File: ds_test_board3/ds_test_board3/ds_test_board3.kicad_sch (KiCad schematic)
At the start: 126 parts, among them J1 DF40C-60DP-0.4V_51_, J2 DF40C-60DP-0.4V_51_, J3 Conn_01x30, J4 Conn_01x30, J5 Conn_01x30, J6 Conn_01x30

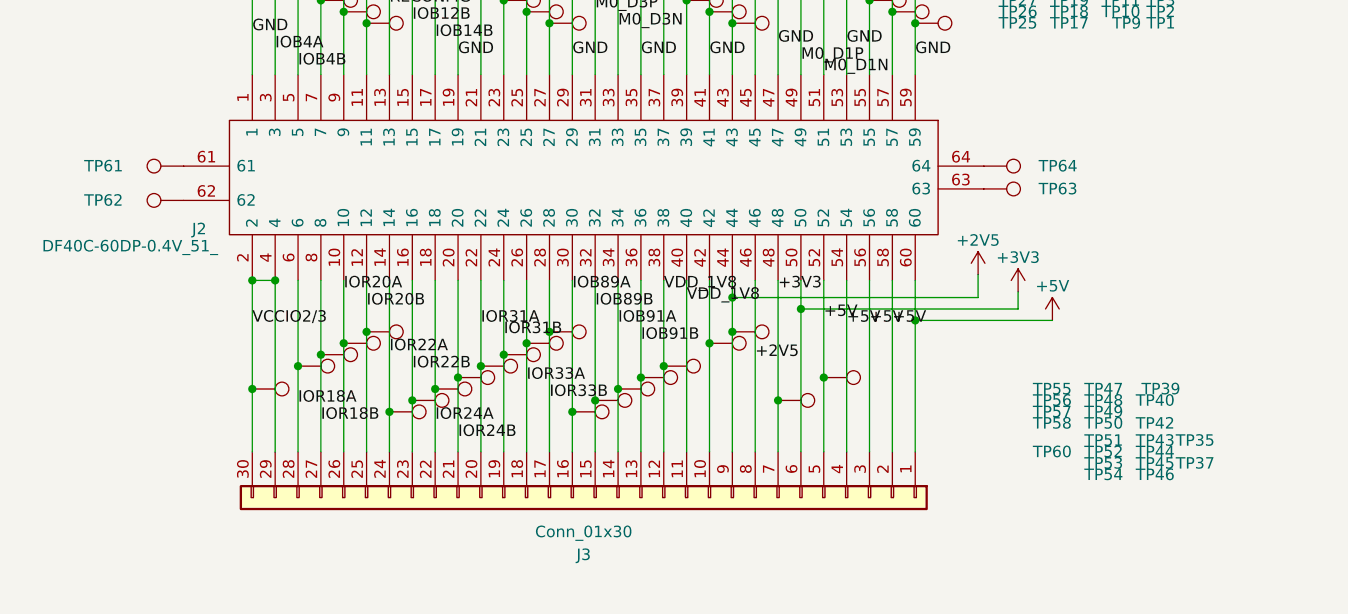
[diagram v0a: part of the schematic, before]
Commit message: 1204
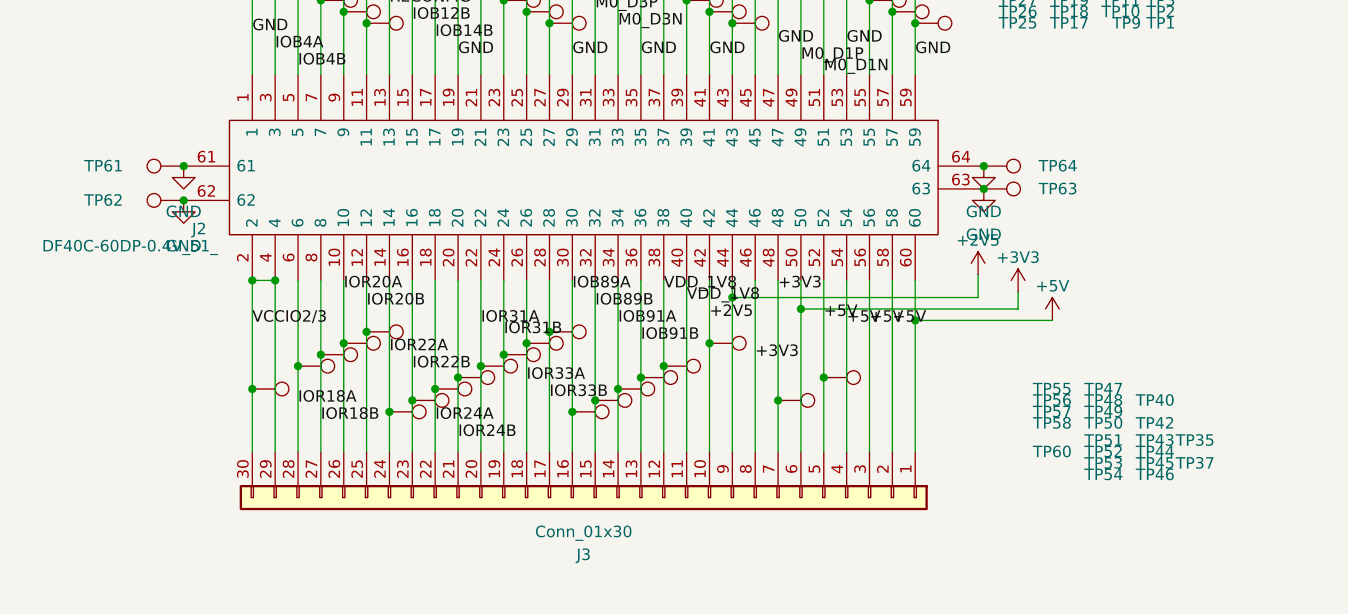
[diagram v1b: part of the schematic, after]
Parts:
- removed TP39: TestPoint, TestPoint:TestPoint_Pad_1.5x1.5mm, symbol Connector:TestPoint
- TP1, TP10, TP11, TP12, TP13, TP14, TP15, TP16, TP17, TP18, TP19, TP2, TP20, TP21, TP22, TP23, TP24, TP25, TP26, TP27, TP28, TP29, TP3, TP30, TP4, TP5, TP6, TP61, TP63, TP7, TP8, TP9: footprint TestPoint:TestPoint_Pad_1.5x1.5mm -> TestPoint:TestPoint_THTPad_1.5x1.5mm_Drill0.7mm
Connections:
- net +2V5: now also J2.42, J3.10 (Pin_10), TP40.1; no longer J2.46, J3.8 (Pin_8)
- net +3V3: now also J2.46, J3.8 (Pin_8)
- net GND: now also J2.61, J2.62, J2.63, J2.64, TP61.1, TP62.1, TP63.1, TP64.1
